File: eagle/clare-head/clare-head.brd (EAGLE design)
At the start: 50 x 70 mm, 22 parts

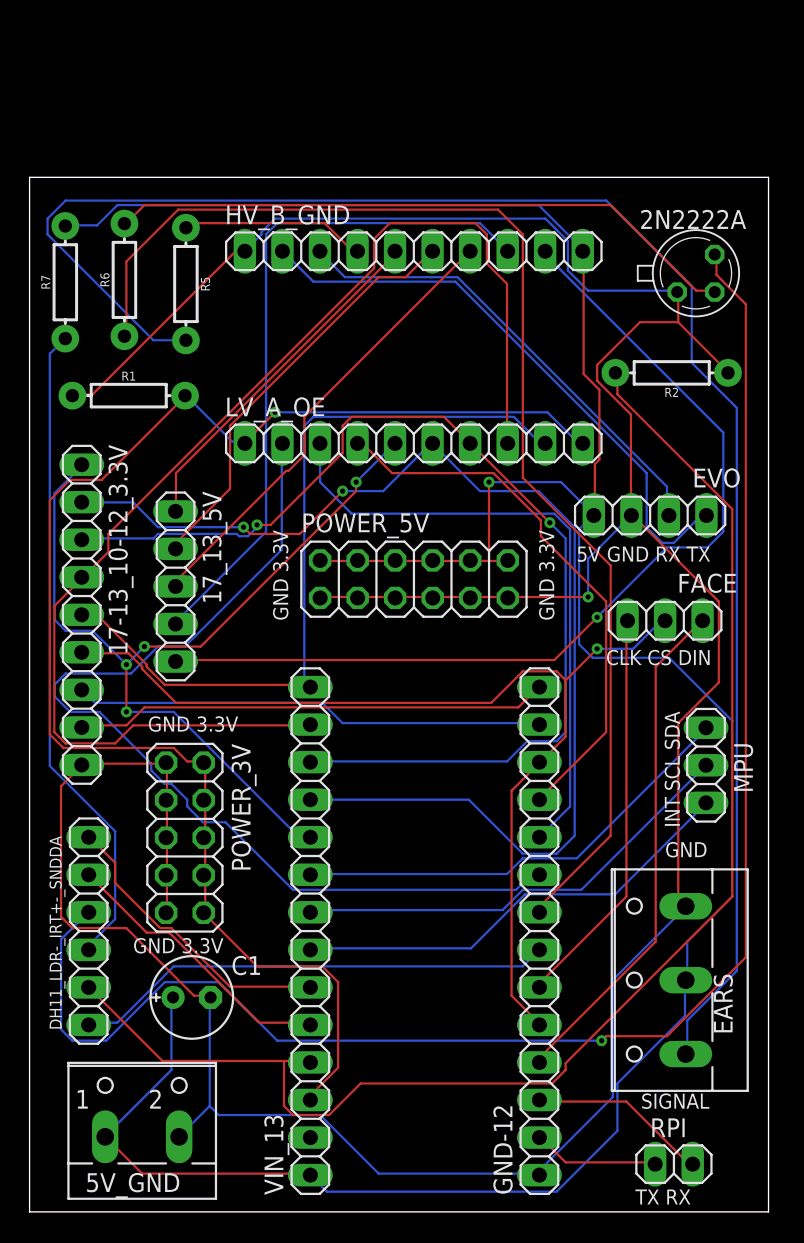
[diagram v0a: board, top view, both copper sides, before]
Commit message: 3d pcb version
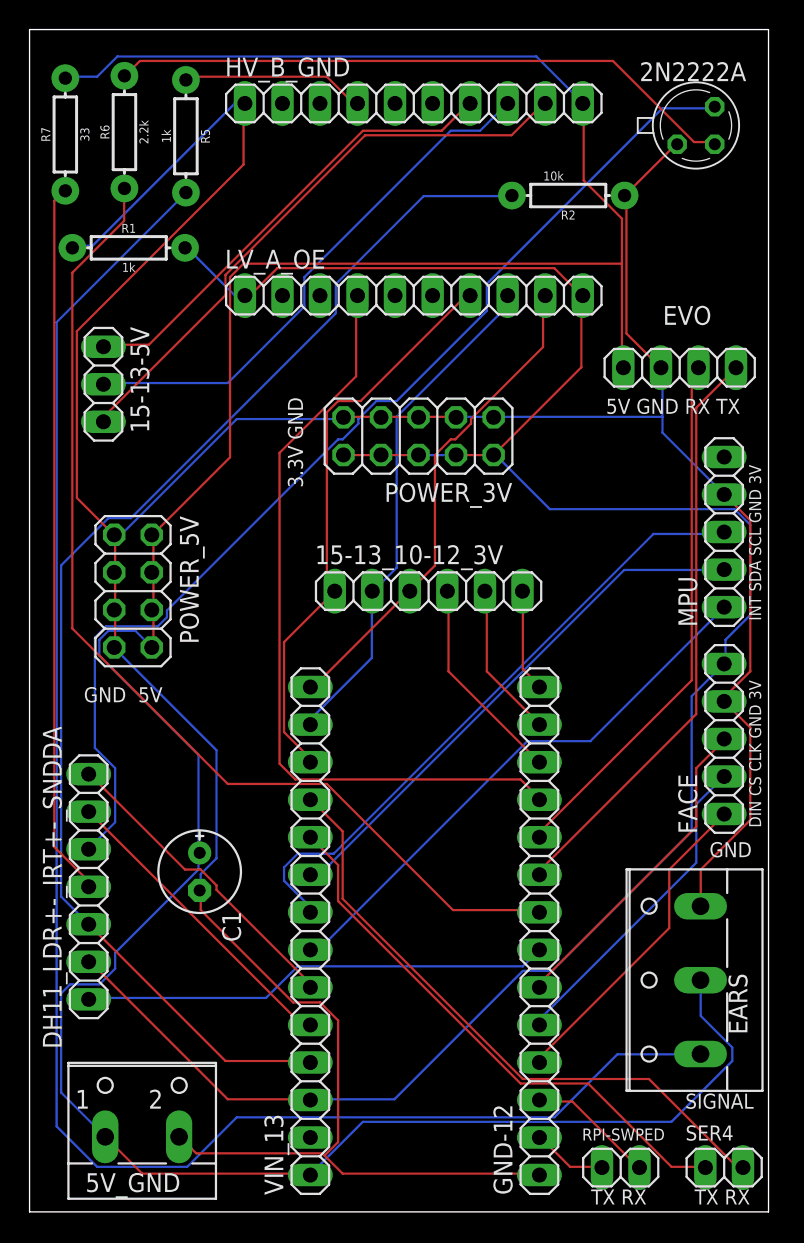
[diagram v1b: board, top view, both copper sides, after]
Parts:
- removed 17-13_10-12_3.3V: (no value), pinhead:1X09
- removed 17_13_5V: (no value), pinhead:1X05
- removed DH11_LDR-_IRT+-_SNDDA: (no value), pinhead:1X06
- removed RPI: (no value), pinhead:1X02
- added 15-13-5V: (no value), pinhead:1X03
- added 15-13_10-12_3V: (no value), pinhead:1X06
- added DH11_LDR+-_IRT+-_SNDDA: (no value), pinhead:1X07
- added RPI-SWPED, SER4: (no value), pinhead:1X02
- FACE, MPU: device pinhead:1X03 -> pinhead:1X05
- POWER_5V: device pinhead:2X06 -> pinhead:2X04
- moved POWER_3V 31.4 mm to (26.3, 52.5), turned to 180 degrees
- moved POWER_5V 19.0 mm to (7.00, 42.0), turned to 270 degrees
- moved MPU 15.8 mm to (47.0, 46.0)
- moved R2 13.9 mm to (36.5, 68.8)
- moved EVO 10.2 mm to (44.0, 57.1)
- moved 2N2222A 10.0 mm to (45.1, 73.5)
- moved R1 10.0 mm to (6.71, 65.2)
- moved R7 10.0 mm to (2.42, 72.9)
- moved HV_B_GND 10.0 mm to (26.0, 75.0)
- moved LV_A_OE 10.0 mm to (26.0, 62.0)
- moved R5 10.0 mm to (10.6, 72.8)
- moved R6 10.0 mm to (6.42, 73.1)
- moved FACE 8.94 mm to (47.0, 32.0), turned to 90 degrees
- moved C1 8.53 mm to (11.5, 23.0), turned to 270 degrees
- moved EARS 1.00 mm to (44.1, 15.7)
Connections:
- removed net N$12: 17-13_10-12_3.3V.1, LV_A_OE.5, VIN_13.10
- removed net N$13: 17-13_10-12_3.3V.2, LV_A_OE.6, VIN_13.11
- removed net N$5: 17_13_5V.1, HV_B_GND.5
- removed net N$6: 17_13_5V.2, HV_B_GND.6
- removed net RXEVO5: EVO.2, HV_B_GND.3
- removed net TXEVO5: EVO.1, HV_B_GND.2
- new net 5V: MPU.5
- new net FCS: FACE.2, GND-12.5
- new net RX4: SER4.2, VIN_13.11
- new net TX4: SER4.1, VIN_13.10
- net +5V: no longer POWER_5V.10, POWER_5V.12
- net 3.3V: now also DH11_LDR+-_IRT+-_SNDDA.2, FACE.5
- net CS: now also 15-13_10-12_3V.4; no longer 17-13_10-12_3.3V.6, FACE.2, GND-12.5
- net DH11: now also DH11_LDR+-_IRT+-_SNDDA.1; no longer DH11_LDR-_IRT+-_SNDDA.1
- net GND: now also FACE.4, MPU.4; no longer 17-13_10-12_3.3V.9, POWER_5V.11, POWER_5V.9
- net IRT+: now also DH11_LDR+-_IRT+-_SNDDA.4; no longer DH11_LDR-_IRT+-_SNDDA.3
- net IRT-: now also DH11_LDR+-_IRT+-_SNDDA.5; no longer DH11_LDR-_IRT+-_SNDDA.4
- net LDR-: now also DH11_LDR+-_IRT+-_SNDDA.3; no longer DH11_LDR-_IRT+-_SNDDA.2
- net MISO: now also 15-13_10-12_3V.6; no longer 17-13_10-12_3.3V.8
- net MOSI: now also 15-13_10-12_3V.5; no longer 17-13_10-12_3.3V.7
- net MPUSCL: now also MPU.3; no longer MPU.2
- net MPUSDA: now also MPU.2; no longer MPU.3
- net N$10: now also 15-13-5V.3; no longer 17_13_5V.5
- net N$14: now also 15-13_10-12_3V.1; no longer 17-13_10-12_3.3V.3
- net N$15: now also 15-13_10-12_3V.2; no longer 17-13_10-12_3.3V.4
- net N$16: now also 15-13_10-12_3V.3; no longer 17-13_10-12_3.3V.5
- net N$7: now also 15-13-5V.1; no longer 17_13_5V.3
- net N$9: now also 15-13-5V.2; no longer 17_13_5V.4
- net RX: now also RPI-SWPED.2; no longer RPI.2
- net RXEVO: now also EVO.2; no longer LV_A_OE.3
- net SND_A: now also DH11_LDR+-_IRT+-_SNDDA.7; no longer DH11_LDR-_IRT+-_SNDDA.6
- net SND_D: now also DH11_LDR+-_IRT+-_SNDDA.6; no longer DH11_LDR-_IRT+-_SNDDA.5
- net TX: now also RPI-SWPED.1; no longer RPI.1
- net TXEVO: now also EVO.1; no longer LV_A_OE.2
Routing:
- net N$13: track 79.9 -> 0.00 mm, vias 2 -> 0
- net N$12: track 61.3 -> 0.00 mm, vias 4 -> 0
- net CS: track 69.4 -> 14.1 mm, vias 1 -> 0
- net N$15: track 83.6 -> 34.6 mm
- net 3.3V: track 99.7 -> 147.1 mm, vias 1 -> 0
- net RX4: track 0.00 -> 42.2 mm
- net TXEVO5: track 39.8 -> 0.00 mm
- net TX4: track 0.00 -> 37.4 mm
- net IRT-: track 109.5 -> 74.0 mm, vias 1 -> 0
- net N$14: track 72.1 -> 39.0 mm, vias 2 -> 0
- net RXEVO5: track 32.1 -> 0.00 mm
- net N$6: track 28.4 -> 0.00 mm
- net +5V: track 183.6 -> 210.7 mm, vias 1 -> 0
- net TXEVO: track 66.4 -> 39.8 mm
- net MISO: track 32.1 -> 6.95 mm
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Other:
- board size 50 x 70 mm -> 50 x 80 mm
- board text added: "3.3V GND"
- board text added: "DIN CS CLK GND 3V"
- board text added: "GND 5V"
- board text added: "INT SDA SCL GND 3V"
- board text removed: "CLK CS DIN"
- board text removed: "GND 3.3V"
- board text removed: "INT SCL SDA"
